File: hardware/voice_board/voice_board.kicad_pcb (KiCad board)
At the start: 2 copper layers, 130 parts, among them J1 Conn_02x06_Odd_Even, J2 Conn_02x02_Odd_Even, J3 Conn_02x02_Odd_Even, J4 Conn_01x02_Male, J5 Conn_02x03_Odd_Even, J6 Conn_02x02_Odd_Even, J7 Conn_02x02_Odd_Even, J8 Conn_02x03_Odd_Even, J9 Conn_02x02_Odd_Even, Q1 BC327, Q10 BC557, Q11 BC557, Q12 BC557, Q13 BC557, Q14 BC557, Q15 BC557, Q16 BC557, Q17 BC547, Q18 BC547, Q19 2N7000, Q2 BC557, Q20 2N7000, Q21 BC547, Q22 BC547, Q3 BC327, Q4 BC557, Q5 BC557, Q6 BC557, Q7 BC557, Q8 BC557, Q9 BC557, U1 TL074, U2 MCP4822, U3 LM324

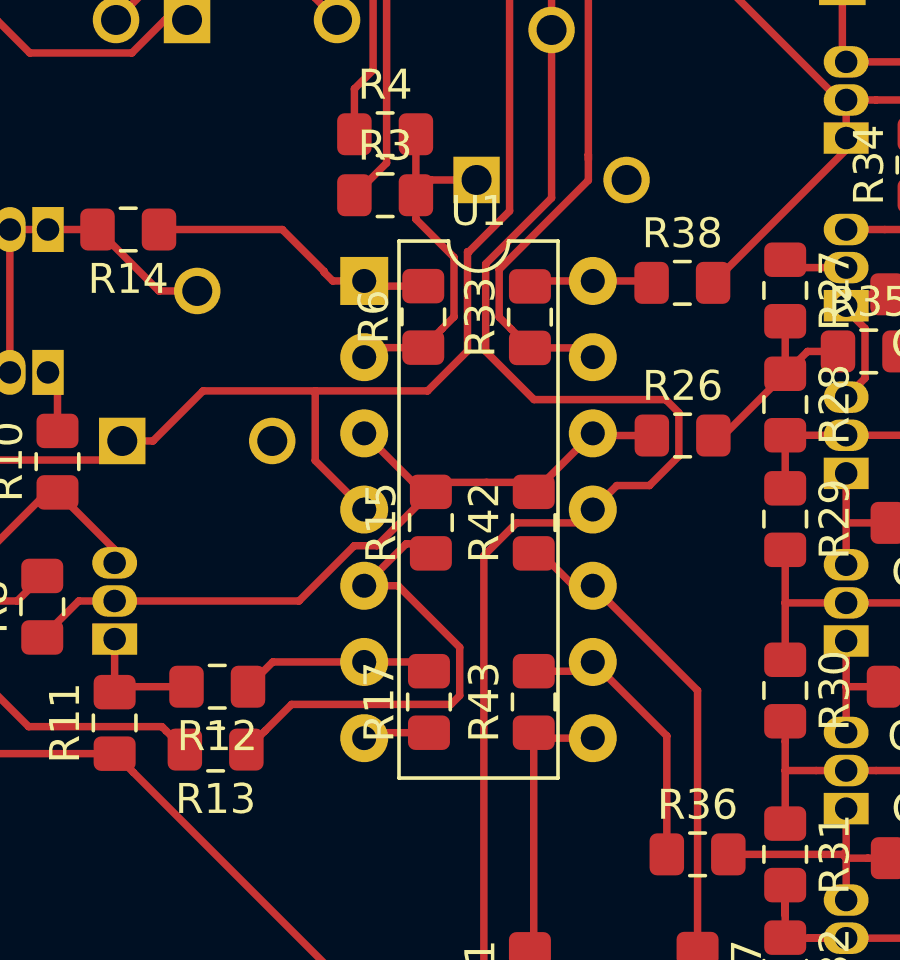
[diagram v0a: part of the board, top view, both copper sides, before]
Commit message: flip footprint
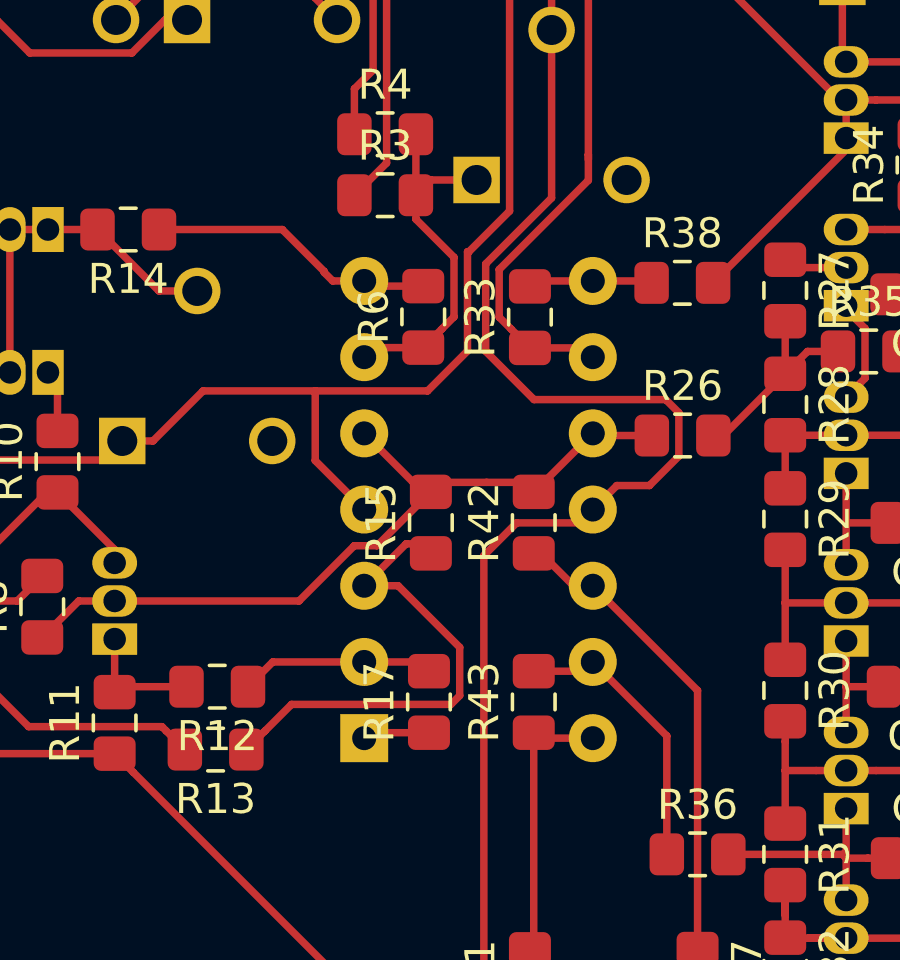
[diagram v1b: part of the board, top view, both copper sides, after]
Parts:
- U1: moved to B.Cu
- moved U1 15.2 mm to (212.9, 69.4)
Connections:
- U1 pad 1: Net-(R14-Pad1) -> Net-(R17-Pad1)
- U1 pad 10: Net-(R37-Pad1) -> GND
- U1 pad 12: GND -> Net-(R37-Pad1)
- U1 pad 13: vcf_ctl_raw -> Net-(R36-Pad1)
- U1 pad 14: Net-(R33-Pad2) -> vcf_audio_out
- U1 pad 2: vca_ctl_raw -> Net-(R12-Pad1)
- U1 pad 3: GND -> Net-(R13-Pad1)
- U1 pad 5: Net-(R13-Pad1) -> GND
- U1 pad 6: Net-(R12-Pad1) -> vca_ctl_raw
- U1 pad 7: Net-(R17-Pad1) -> Net-(R14-Pad1)
- U1 pad 8: vcf_audio_out -> Net-(R33-Pad2)
- U1 pad 9: Net-(R36-Pad1) -> vcf_ctl_raw
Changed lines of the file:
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@@
     )
   )
-  (module Package_DIP:DIP-14_W7.62mm (layer F.Cu)
-    (at 212.9155 54.1655)
+  (module Package_DIP:DIP-14_W7.62mm (layer B.Cu)
+    (at 212.9155 69.4055)
     (descr "14-lead though-hole mounted DIP package, row spacing 7.62 mm (300 mils)")
     (tags "THT DIP DIL PDIP 2.54mm 7.62mm 300mil")
-    (fp_text reference U1 (at 3.81 -2.33 180) (layer F.SilkS)
-      (effects (font (size 1 1) (thickness 0.15)))
+    (fp_text reference U1 (at 3.81 2.33 -180) (layer B.SilkS)
+      (effects (font (size 1 1) (thickness 0.15)) (justify mirror))
     )
-    (fp_text value TL074 (at 3.81 17.57 180) (layer F.Fab)
-      (effects (font (size 1 1) (thickness 0.15)))
+    (fp_text value TL074 (at 3.81 -17.57 -180) (layer B.Fab)
+      (effects (font (size 1 1) (thickness 0.15)) (justify mirror))
     )
-    (fp_text user %R (at 4.699 9.5885 180) (layer F.Fab)
-      (effects (font (size 1 1) (thickness 0.15)))
+    (fp_text user %R (at 4.699 -9.5885 -180) (layer B.Fab)
+      (effects (font (size 1 1) (thickness 0.15)) (justify mirror))
     )
-    (fp_line (start 8.7 -1.55) (end -1.1 -1.55) (layer F.CrtYd) (width 0.05))
-    (fp_line (start 8.7 16.8) (end 8.7 -1.55) (layer F.CrtYd) (width 0.05))
-    (fp_line (start -1.1 16.8) (end 8.7 16.8) (layer F.CrtYd) (width 0.05))
-    (fp_line (start -1.1 -1.55) (end -1.1 16.8) (layer F.CrtYd) (width 0.05))
-    (fp_line (start 6.46 -1.33) (end 4.81 -1.33) (layer F.SilkS) (width 0.12))
-    (fp_line (start 6.46 16.57) (end 6.46 -1.33) (layer F.SilkS) (width 0.12))
-    (fp_line (start 1.16 16.57) (end 6.46 16.57) (layer F.SilkS) (width 0.12))
-    (fp_line (start 1.16 -1.33) (end 1.16 16.57) (layer F.SilkS) (width 0.12))
-    (fp_line (start 2.81 -1.33) (end 1.16 -1.33) (layer F.SilkS) (width 0.12))
-    (fp_line (start 0.635 -0.27) (end 1.635 -1.27) (layer F.Fab) (width 0.1))
-    (fp_line (start 0.635 16.51) (end 0.635 -0.27) (layer F.Fab) (width 0.1))
-    (fp_line (start 6.985 16.51) (end 0.635 16.51) (layer F.Fab) (width 0.1))
-    (fp_line (start 6.985 -1.27) (end 6.985 16.51) (layer F.Fab) (width 0.1))
-    (fp_line (start 1.635 -1.27) (end 6.985 -1.27) (layer F.Fab) (width 0.1))
-    (fp_arc (start 3.81 -1.33) (end 2.81 -1.33) (angle -180) (layer F.SilkS) (width 0.12))
+    (fp_line (start 8.7 1.55) (end -1.1 1.55) (layer B.CrtYd) (width 0.05))
+    (fp_line (start 8.7 -16.8) (end 8.7 1.55) (layer B.CrtYd) (width 0.05))
+    (fp_line (start -1.1 -16.8) (end 8.7 -16.8) (layer B.CrtYd) (width 0.05))
+    (fp_line (start -1.1 1.55) (end -1.1 -16.8) (layer B.CrtYd) (width 0.05))
+    (fp_line (start 6.46 1.33) (end 4.81 1.33) (layer B.SilkS) (width 0.12))
+    (fp_line (start 6.46 -16.57) (end 6.46 1.33) (layer B.SilkS) (width 0.12))
+    (fp_line (start 1.16 -16.57) (end 6.46 -16.57) (layer B.SilkS) (width 0.12))
+    (fp_line (start 1.16 1.33) (end 1.16 -16.57) (layer B.SilkS) (width 0.12))
+    (fp_line (start 2.81 1.33) (end 1.16 1.33) (layer B.SilkS) (width 0.12))
+    (fp_line (start 0.635 0.27) (end 1.635 1.27) (layer B.Fab) (width 0.1))
+    (fp_line (start 0.635 -16.51) (end 0.635 0.27) (layer B.Fab) (width 0.1))
+    (fp_line (start 6.985 -16.51) (end 0.635 -16.51) (layer B.Fab) (width 0.1))
+    (fp_line (start 6.985 1.27) (end 6.985 -16.51) (layer B.Fab) (width 0.1))
+    (fp_line (start 1.635 1.27) (end 6.985 1.27) (layer B.Fab) (width 0.1))
+    (fp_arc (start 3.81 1.33) (end 2.81 1.33) (angle 180) (layer B.SilkS) (width 0.12))
     (pad 14 thru_hole oval (at 7.62 0) (size 1.6 1.6) (drill 0.8) (layers *.Cu *.Mask)
+      (net 76 vcf_audio_out))
+    (pad 7 thru_hole oval (at 0 -15.24) (size 1.6 1.6) (drill 0.8) (layers *.Cu *.Mask)
+      (net 64 "Net-(R14-Pad1)"))
+    (pad 13 thru_hole oval (at 7.62 -2.54) (size 1.6 1.6) (drill 0.8) (layers *.Cu *.Mask)
+      (net 73 "Net-(R36-Pad1)"))
+    (pad 6 thru_hole oval (at 0 -12.7) (size 1.6 1.6) (drill 0.8) (layers *.Cu *.Mask)
+      (net 63 vca_ctl_raw))
+    (pad 12 thru_hole oval (at 7.62 -5.08) (size 1.6 1.6) (drill 0.8) (layers *.Cu *.Mask)
+      (net 74 "Net-(R37-Pad1)"))
+    (pad 5 thru_hole oval (at 0 -10.16) (size 1.6 1.6) (drill 0.8) (layers *.Cu *.Mask)
+      (net 19 GND))
+    (pad 11 thru_hole oval (at 7.62 -7.62) (size 1.6 1.6) (drill 0.8) (layers *.Cu *.Mask)
+      (net 37 VEE))
+    (pad 4 thru_hole oval (at 0 -7.62) (size 1.6 1.6) (drill 0.8) (layers *.Cu *.Mask)
+      (net 38 VCC))
+    (pad 10 thru_hole oval (at 7.62 -10.16) (size 1.6 1.6) (drill 0.8) (layers *.Cu *.Mask)
+      (net 19 GND))
+    (pad 3 thru_hole oval (at 0 -5.08) (size 1.6 1.6) (drill 0.8) (layers *.Cu *.Mask)
+      (net 66 "Net-(R13-Pad1)"))
+    (pad 9 thru_hole oval (at 7.62 -12.7) (size 1.6 1.6) (drill 0.8) (layers *.Cu *.Mask)
+      (net 70 vcf_ctl_raw))
+    (pad 2 thru_hole oval (at 0 -2.54) (size 1.6 1.6) (drill 0.8) (layers *.Cu *.Mask)
+      (net 65 "Net-(R12-Pad1)"))
+    (pad 8 thru_hole oval (at 7.62 -15.24) (size 1.6 1.6) (drill 0.8) (layers *.Cu *.Mask)
       (net 72 "Net-(R33-Pad2)"))
-    (pad 7 thru_hole oval (at 0 15.24) (size 1.6 1.6) (drill 0.8) (layers *.Cu *.Mask)
+    (pad 1 thru_hole rect (at 0 0) (size 1.6 1.6) (drill 0.8) (layers *.Cu *.Mask)
       (net 98 "Net-(R17-Pad1)"))
-    (pad 13 thru_hole oval (at 7.62 2.54) (size 1.6 1.6) (drill 0.8) (layers *.Cu *.Mask)
-      (net 70 vcf_ctl_raw))
-    (pad 6 thru_hole oval (at 0 12.7) (size 1.6 1.6) (drill 0.8) (layers *.Cu *.Mask)
-      (net 65 "Net-(R12-Pad1)"))
-    (pad 12 thru_hole oval (at 7.62 5.08) (size 1.6 1.6) (drill 0.8) (layers *.Cu *.Mask)
-      (net 19 GND))
-    (pad 5 thru_hole oval (at 0 10.16) (size 1.6 1.6) (drill 0.8) (layers *.Cu *.Mask)
-      (net 66 "Net-(R13-Pad1)"))
-    (pad 11 thru_hole oval (at 7.62 7.62) (size 1.6 1.6) (drill 0.8) (layers *.Cu *.Mask)
-      (net 37 VEE))
-    (pad 4 thru_hole oval (at 0 7.62) (size 1.6 1.6) (drill 0.8) (layers *.Cu *.Mask)
-      (net 38 VCC))
-    (pad 10 thru_hole oval (at 7.62 10.16) (size 1.6 1.6) (drill 0.8) (layers *.Cu *.Mask)
-      (net 74 "Net-(R37-Pad1)"))
-    (pad 3 thru_hole oval (at 0 5.08) (size 1.6 1.6) (drill 0.8) (layers *.Cu *.Mask)
-      (net 19 GND))
-    (pad 9 thru_hole oval (at 7.62 12.7) (size 1.6 1.6) (drill 0.8) (layers *.Cu *.Mask)
-      (net 73 "Net-(R36-Pad1)"))
-    (pad 2 thru_hole oval (at 0 2.54) (size 1.6 1.6) (drill 0.8) (layers *.Cu *.Mask)
-      (net 63 vca_ctl_raw))
-    (pad 8 thru_hole oval (at 7.62 15.24) (size 1.6 1.6) (drill 0.8) (layers *.Cu *.Mask)
-      (net 76 vcf_audio_out))
-    (pad 1 thru_hole rect (at 0 0) (size 1.6 1.6) (drill 0.8) (layers *.Cu *.Mask)
-      (net 64 "Net-(R14-Pad1)"))
     (model ${KISYS3DMOD}/Package_DIP.3dshapes/DIP-14_W7.62mm.wrl
       (at (xyz 0 0 0))
